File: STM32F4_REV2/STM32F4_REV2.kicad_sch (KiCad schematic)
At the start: 50 parts, among them J1 Screw_Terminal_01x02, J2 SWD, J3 Conn_01x04, J4 Conn_01x04, J5 USB_B_Micro, Q1 AO3401A, SW1 SW_SPDT, U1 STM32F405RGT6, U3 USBLC6-2SC6, Y1 16MHz

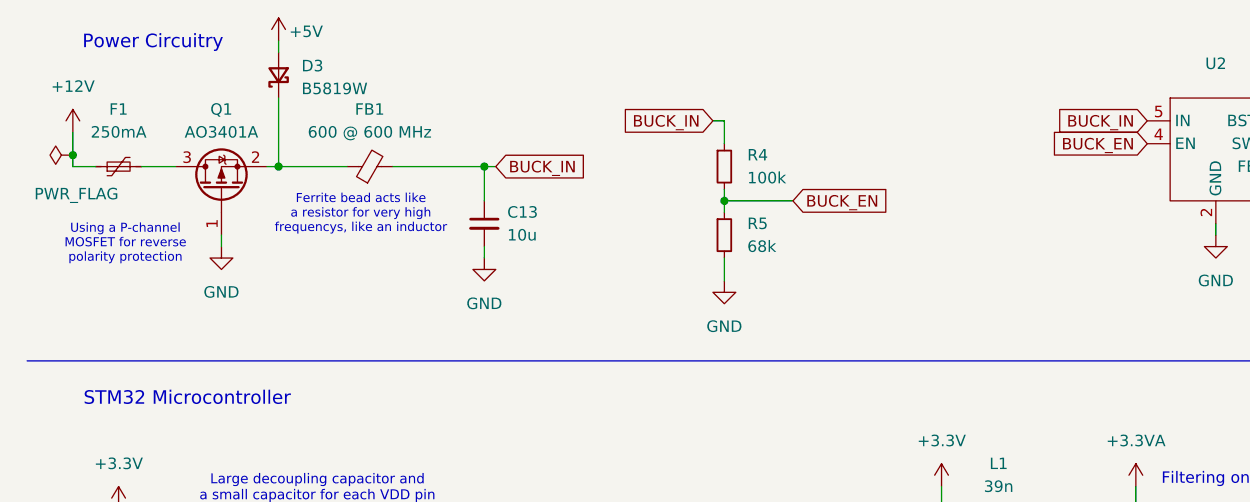
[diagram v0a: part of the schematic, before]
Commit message: Layout finished
Finished the layout, need to route
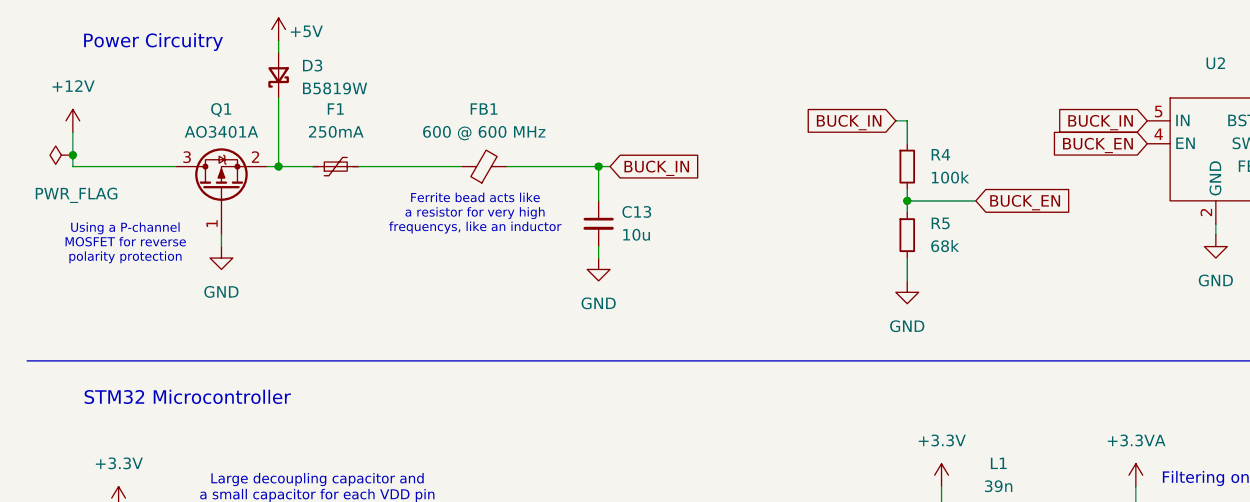
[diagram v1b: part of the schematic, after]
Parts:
- C10: footprint Capacitor_SMD:C_0603_1608Metric -> Capacitor_SMD:C_0402_1005Metric
- J5: footprint Connector_USB:USB_Micro-B_Amphenol_10118194_Horizontal -> Connector_USB:USB_Micro-B_Amphenol_10118193-0001LF_Horizontal
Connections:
- net +12V: now also Q1.3 (D); no longer F1.1
- net at D3.1 (K), Q1.2 (S): now also F1.1; no longer FB1.1
- net at F1.2: now also FB1.1; no longer Q1.3 (D)
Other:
- moved on the sheet: C13, F1, FB1, R4, R5
